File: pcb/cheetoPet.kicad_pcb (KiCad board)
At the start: 2 copper layers, 34.2 x 53.6 mm, 35 parts, among them J1 SH1107 Display 128x128, J4 Conn_02x06_Counter_Clockwise, P1 USB_C_Plug_USB2.0, SW1 B, SW2 X, SW3 A, SW4 SW_Push_SPDT, SW5 RESET, SW6 BOOT, U1 DS3231M, U2 MPU-9250, U3 TP4056-42-ESOP8, U4 ESP32-C3-WROOM-02U, U5 ADS1115IDGS, U7 AT24CS04-SSHM, U8 MCP1700x-330xxTT

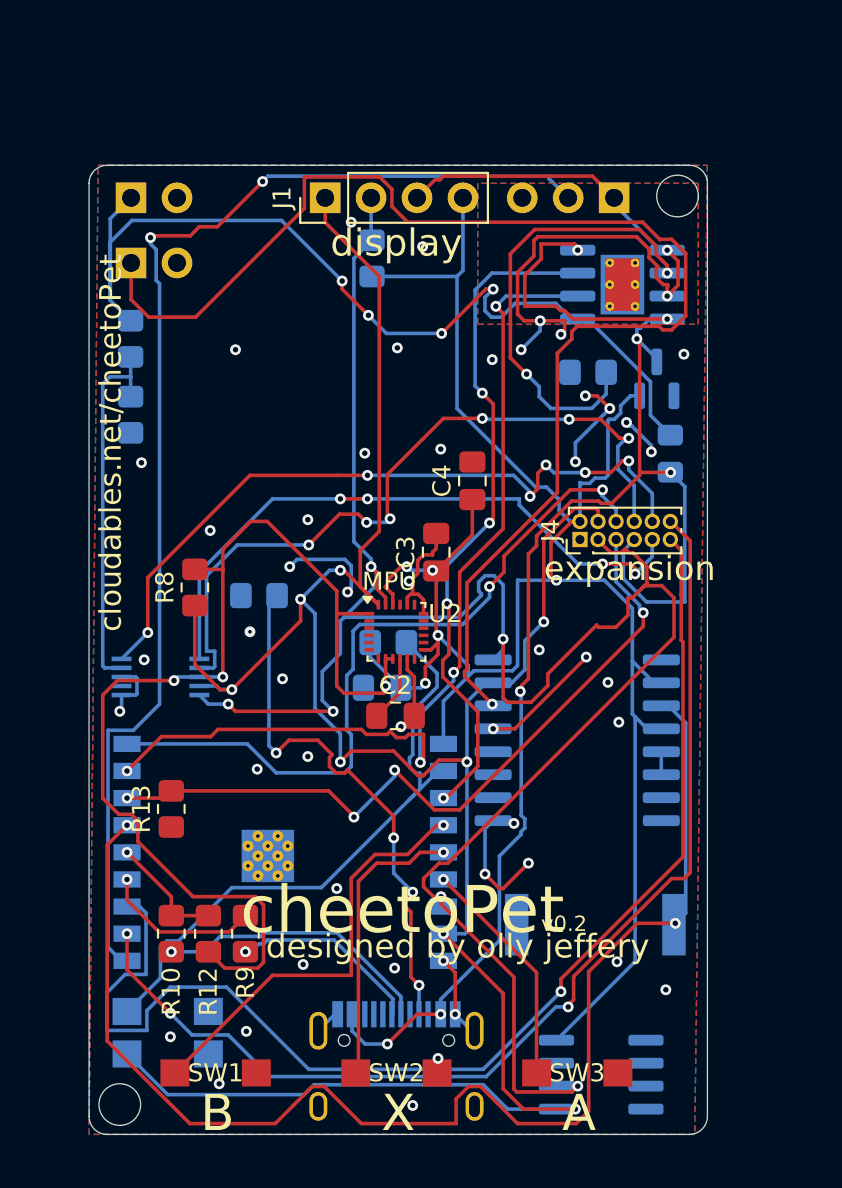
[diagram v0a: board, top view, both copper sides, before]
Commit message: NEW PCB v0.3, pretty much finished, also some code changes (i think safe crack game which is rubbish)
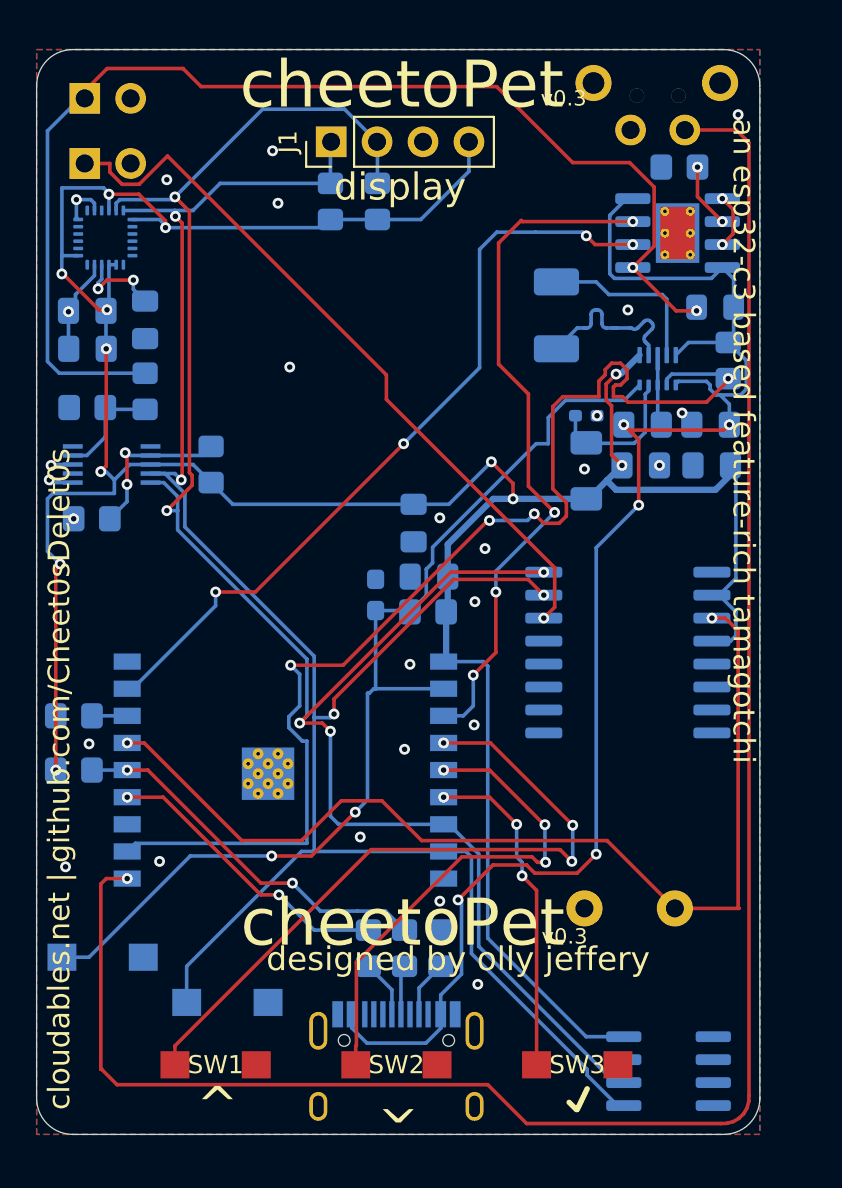
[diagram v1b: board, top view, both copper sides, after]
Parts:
- removed J4: Conn_02x06_Counter_Clockwise, Connector_PinHeader_1.00mm:PinHeader_2x06_P1.00mm_Vertical
- removed U8: MCP1700x-330xxTT, Package_TO_SOT_SMD:SOT-23
- added C10: 10µF, Capacitor_SMD:C_0805_2012Metric_Pad1.18x1.45mm_HandSolder, B.Cu at (159.2, 95.4)
- added C5: 10µF, Capacitor_SMD:C_0805_2012Metric_Pad1.18x1.45mm_HandSolder, B.Cu at (171.9, 90.0)
- added C6: 10µF, Capacitor_SMD:C_0805_2012Metric_Pad1.18x1.45mm_HandSolder, B.Cu at (175.7, 90.0)
- added C7: 22µF, Capacitor_SMD:C_0805_2012Metric_Pad1.18x1.45mm_HandSolder, B.Cu at (171.8, 92.2)
- added C8: 22µF, Capacitor_SMD:C_0805_2012Metric_Pad1.18x1.45mm_HandSolder, B.Cu at (175.7, 92.2)
- added C9: 100nF, Capacitor_SMD:C_0603_1608Metric_Pad1.08x0.95mm_HandSolder, B.Cu at (157.2, 99.4)
- added L1: 1 µH, Inductor_SMD:L_Changjiang_FXL0420, B.Cu at (167.2, 83.9)
- added R14: 100k, Resistor_SMD:R_0805_2012Metric_Pad1.20x1.40mm_HandSolder, B.Cu at (148.1, 92.2)
- added R15: 100k, Resistor_SMD:R_0805_2012Metric_Pad1.20x1.40mm_HandSolder, B.Cu at (141.4, 95.2)
- added R16: 100k, Resistor_SMD:R_0805_2012Metric_Pad1.20x1.40mm_HandSolder, B.Cu at (176.7, 86.4)
- added R3: 1M, Resistor_SMD:R_1206_3216Metric_Pad1.30x1.75mm_HandSolder, B.Cu at (168.8, 92.5)
- added R4: 309k, Resistor_SMD:R_0402_1005Metric_Pad0.72x0.64mm_HandSolder, B.Cu at (168.8, 89.5)
- added U6: TPS63802DLAR, cheeto:VREG_TPS63802DLAR, B.Cu at (172.8, 86.8)
- C2, C3, C4, R10, R12, R13, R8, R9, U2: moved to B.Cu
- LS1: footprint Buzzer_Beeper:Buzzer_Murata_PKMCS0909E -> cheeto:PS1240_PassiveBuzzer_12.2x3.5mm
- SW4: value SW_Push_SPDT -> POWER; footprint Connector_PinHeader_2.54mm:PinHeader_1x03_P2.54mm_Horizontal -> cheeto:side switch
- moved U2 27.1 mm to (142.2, 79.6), turned to 180 degrees
- moved C2 25.9 mm to (144.4, 84.2), turned to -90 degrees
- moved C4 23.3 mm to (141.2, 83.7), turned to 180 degrees
- moved R8 22.6 mm to (154.7, 77.6), turned to -90 degrees
- moved C3 22.3 mm to (141.2, 85.8), turned to 180 degrees
- moved R2 21.9 mm to (160.8, 118.9), turned to 90 degrees
- moved R10 12.9 mm to (158.8, 118.9)
- moved R5 12.4 mm to (173.9, 75.7)
- moved U5 12.1 mm to (142.6, 92.2)
- moved R12 11.7 mm to (140.5, 109.0), turned to 180 degrees
- moved D1 8.47 mm to (175.9, 83.5), turned to 180 degrees
- moved R13 7.45 mm to (140.5, 106.0), turned to 0 degrees
- moved R9 6.85 mm to (156.8, 118.9)
- moved C1 6.67 mm to (160.1, 98.3)
- moved BT1 6.07 mm to (141.1, 71.9)
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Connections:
- net Net-(U4-EN) renamed PG
- SW4 pad 1: GND -> Net-(U4-IO10)
- SW4 pad 2: Net-(SW4-B) -> GND
- SW4 pad 3: unconnected-(SW4-C-Pad3) -> (no net)
- U4 pad 10: Net-(SW4-B) -> Net-(U4-IO10)
- U4 pad 11: RXD -> MODE
- U4 pad 12: TXD -> unconnected-(U4-IO21/TXD-Pad12)
- U5 pad 7: AIN3 -> Net-(U5-AIN3)
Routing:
- net Net-(U4-IO10): track 0.00 -> 106.4 mm, vias 0 -> 1
- net GND: track 88.1 -> 17.3 mm, vias 51 -> 29
- net Net-(SW4-B): track 67.9 -> 0.00 mm, vias 2 -> 0
- net TXD: track 67.8 -> 0.00 mm, vias 1 -> 0
- net MODE: track 0.00 -> 65.8 mm, vias 0 -> 4
- net RXD: track 60.8 -> 0.00 mm, vias 3 -> 0
- net AIN3: track 41.3 -> 0.00 mm, vias 6 -> 0
- net IO0: track 41.1 -> 0.00 mm, vias 2 -> 0
- net AIN1: track 40.5 -> 0.00 mm, vias 6 -> 0
- net IO2: track 41.1 -> 1.95 mm, vias 4 -> 0
- net AIN2: track 35.4 -> 0.00 mm, vias 4 -> 0
- net Net-(BT2-+): track 73.6 -> 40.7 mm
- net Net-(P1-CC): track 30.3 -> 3.15 mm, vias 4 -> 0
- net SDA: track 133.7 -> 111.1 mm, vias 8 -> 4
- net PG: track 34.7 -> 57.3 mm, vias 0 -> 2
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- removed copper zone on B.Cu, net unconnected-(U3-EPAD-Pad9)
- removed copper zone on F.Cu, net unconnected-(U3-EPAD-Pad9)
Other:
- board size 34.2 x 53.6 mm -> 40 x 60 mm
- board text added: "RTC"
- board text added: "^"
- board text added: "an esp32-c3 based feature-rich tamagotchi"
- board text added: "cloudables.net | github.com/Cheet0sDelet0s"
- board text added: "v0.3"
- board text added: "v0.3 olly j."
- board text removed: "A"
- board text removed: "B"
- board text removed: "X"
- board text removed: "cloudables.net/cheetoPet"
- board text removed: "expansion"
- board text removed: "v0.2"
- board text removed: "v0.2 olly j."
